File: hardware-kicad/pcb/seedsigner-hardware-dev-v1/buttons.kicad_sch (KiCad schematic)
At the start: 16 parts, among them SW1 SW_Push, SW2 SW_Push, SW3 SW_Push, SW4 SW_Push, SW5 SW_Push, SW6 SW_Push, SW7 SW_Push, SW8 SW_Push

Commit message: use hierarchical sheets in kicad
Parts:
- R1, R2, R3, R4, R5, R6, R7, R8: footprint Resistor_SMD:R_0603_1608Metric_Pad0.98x0.95mm_HandSolder -> Resistor_SMD:R_0805_2012Metric_Pad1.20x1.40mm_HandSolder
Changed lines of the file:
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@@
 			)
 		)
-		(property "Footprint" "Resistor_SMD:R_0603_1608Metric_Pad0.98x0.95mm_HandSolder"
+		(property "Footprint" "Resistor_SMD:R_0805_2012Metric_Pad1.20x1.40mm_HandSolder"
 			(at 113.538 74.93 90)
 			(effects
@@
 			)
 		)
-		(property "Footprint" "Resistor_SMD:R_0603_1608Metric_Pad0.98x0.95mm_HandSolder"
+		(property "Footprint" "Resistor_SMD:R_0805_2012Metric_Pad1.20x1.40mm_HandSolder"
 			(at 138.938 74.93 90)
 			(effects
@@
 			)
 		)
-		(property "Footprint" "Resistor_SMD:R_0603_1608Metric_Pad0.98x0.95mm_HandSolder"
+		(property "Footprint" "Resistor_SMD:R_0805_2012Metric_Pad1.20x1.40mm_HandSolder"
 			(at 157.988 74.93 90)
 			(effects
@@
 			)
 		)
-		(property "Footprint" "Resistor_SMD:R_0603_1608Metric_Pad0.98x0.95mm_HandSolder"
+		(property "Footprint" "Resistor_SMD:R_0805_2012Metric_Pad1.20x1.40mm_HandSolder"
 			(at 126.238 74.93 90)
 			(effects
@@
 			)
 		)
-		(property "Footprint" "Resistor_SMD:R_0603_1608Metric_Pad0.98x0.95mm_HandSolder"
+		(property "Footprint" "Resistor_SMD:R_0805_2012Metric_Pad1.20x1.40mm_HandSolder"
 			(at 151.638 74.93 90)
 			(effects
@@
 			)
 		)
-		(property "Footprint" "Resistor_SMD:R_0603_1608Metric_Pad0.98x0.95mm_HandSolder"
+		(property "Footprint" "Resistor_SMD:R_0805_2012Metric_Pad1.20x1.40mm_HandSolder"
 			(at 145.288 74.93 90)
 			(effects
@@
 			)
 		)
-		(property "Footprint" "Resistor_SMD:R_0603_1608Metric_Pad0.98x0.95mm_HandSolder"
+		(property "Footprint" "Resistor_SMD:R_0805_2012Metric_Pad1.20x1.40mm_HandSolder"
 			(at 132.588 74.93 90)
 			(effects
@@
 			)
 		)
-		(property "Footprint" "Resistor_SMD:R_0603_1608Metric_Pad0.98x0.95mm_HandSolder"
+		(property "Footprint" "Resistor_SMD:R_0805_2012Metric_Pad1.20x1.40mm_HandSolder"
 			(at 119.888 74.93 90)
 			(effects

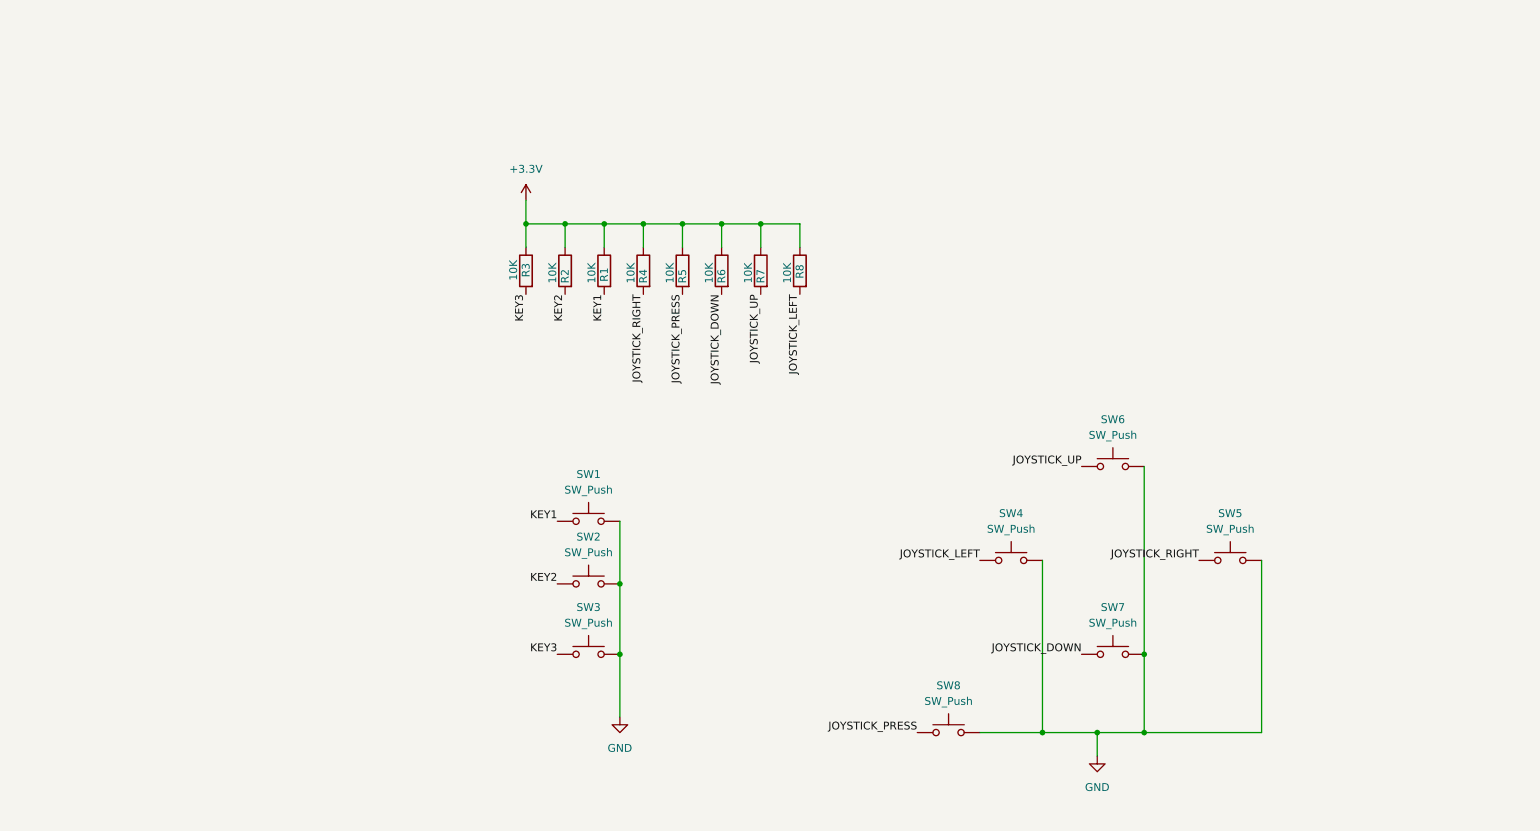
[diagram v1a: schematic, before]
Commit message: 2 different pcbs almost done
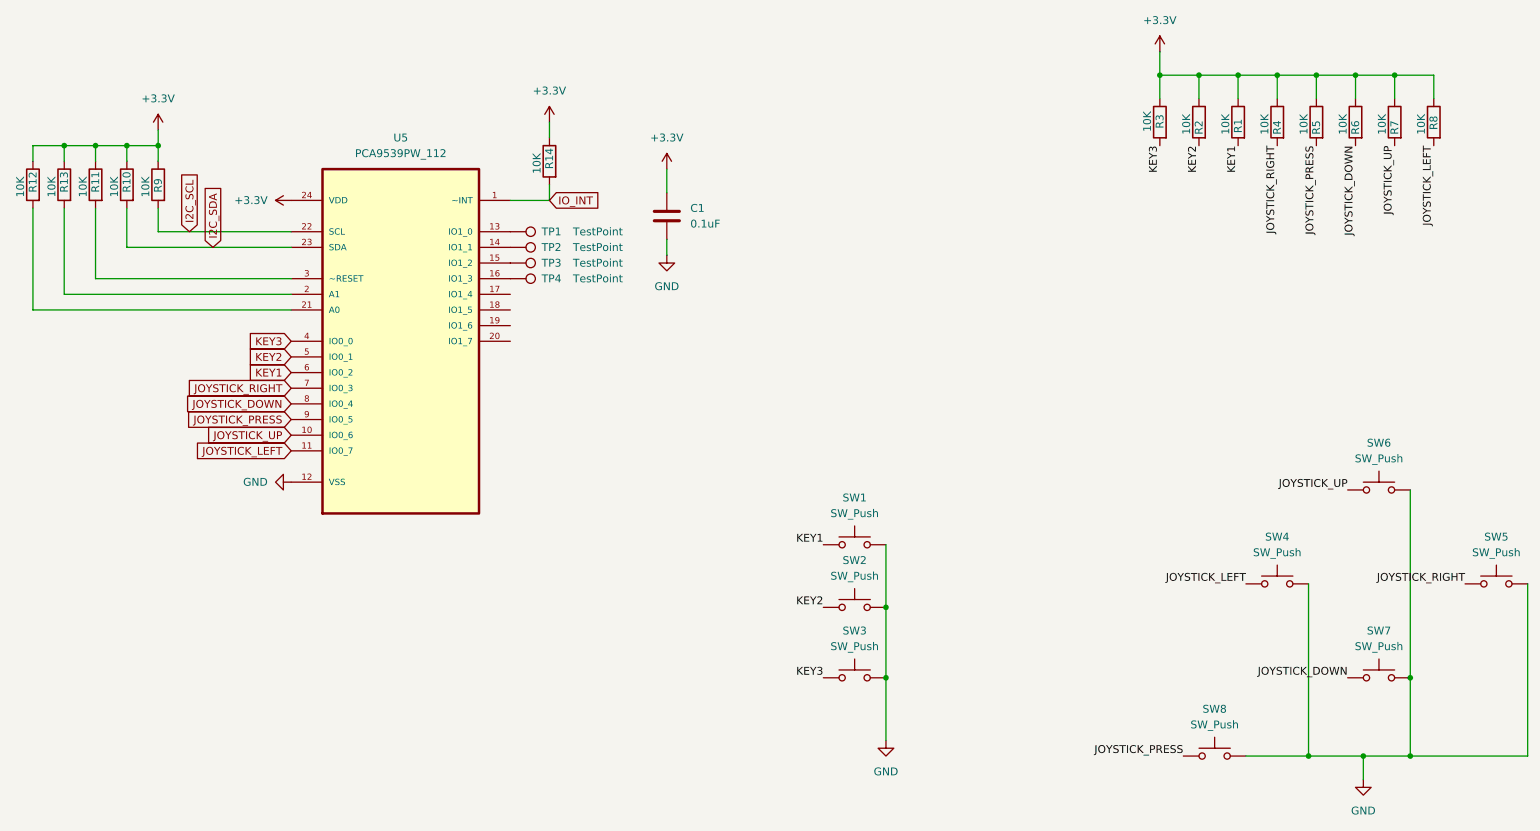
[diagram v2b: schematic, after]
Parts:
- added C1: 0.1uF, Capacitor_SMD:C_0805_2012Metric_Pad1.18x1.45mm_HandSolder, symbol Device:C
- added R10, R11, R12, R13, R14, R9: 10K, Resistor_SMD:R_0805_2012Metric_Pad1.20x1.40mm_HandSolder, symbol Device:R
- added TP1, TP2, TP3, TP4: TestPoint, TestPoint:TestPoint_Pad_D1.0mm, symbol Connector:TestPoint
- added U5: PCA9539PW_112, seedsigner-luckfox:SOP65P640X110-24N, symbol SeedSigner:PCA9539PW_112
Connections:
- net +3.3V: now also C1.1, R10.1, R11.1, R12.1, R13.1, R14.1, R9.1, U5.24 (VDD)
- net GND: now also C1.2, U5.12 (VSS)
- net JOYSTICK_DOWN: now also U5.8 (IO0_4)
- net JOYSTICK_LEFT: now also U5.11 (IO0_7)
- net JOYSTICK_PRESS: now also U5.9 (IO0_5)
- net JOYSTICK_RIGHT: now also U5.7 (IO0_3)
- net JOYSTICK_UP: now also U5.10 (IO0_6)
- net KEY1: now also U5.6 (IO0_2)
- net KEY2: now also U5.5 (IO0_1)
- net KEY3: now also U5.4 (IO0_0)
- new net: TP1.1, U5.13 (IO1_0)
- new net: TP2.1, U5.14 (IO1_1)
- new net: TP3.1, U5.15 (IO1_2)
- new net: TP4.1, U5.16 (IO1_3)
- new net: R13.2, U5.2 (A1)
- new net: R12.2, U5.21 (A0)
- new net: R11.2, U5.3 (~RESET)
- new net I2C_SCL: R9.2, U5.22 (SCL)
- new net I2C_SDA: R10.2, U5.23 (SDA)
- new net IO_INT: R14.2, U5.1 (~INT)
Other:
- moved on the sheet: R1, R2, R3, R4, R5, R6, R7, R8, SW1, SW2, SW3, SW4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
